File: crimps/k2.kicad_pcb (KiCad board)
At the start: 2 copper layers, 99 x 128.5 mm, 100 parts, among them IC1 TL074, IC2 TL072, IC3 TL074, J1 PJ301_THONKICONN6, J10 PJ301_THONKICONN6, J11 PJ301_THONKICONN6, J12 PJ301_THONKICONN6, J13 Conn_01x05_Female, J14 Conn_01x05_Female, J15 Conn_01x05_Female, J16 Conn_01x05_Male, J17 Conn_01x05_Male, J18 Conn_01x05_Male, J2 PJ301_THONKICONN6, J3 PJ301_THONKICONN6, J4 PJ301_THONKICONN6, J5 PJ301_THONKICONN6, J6 PJ301_THONKICONN6, J7 PJ301_THONKICONN6, J8 PJ301_THONKICONN6, J9 PJ301_THONKICONN6, Q1 MMBFJ309, Q2 MMBT3904, Q3 MMBT3904

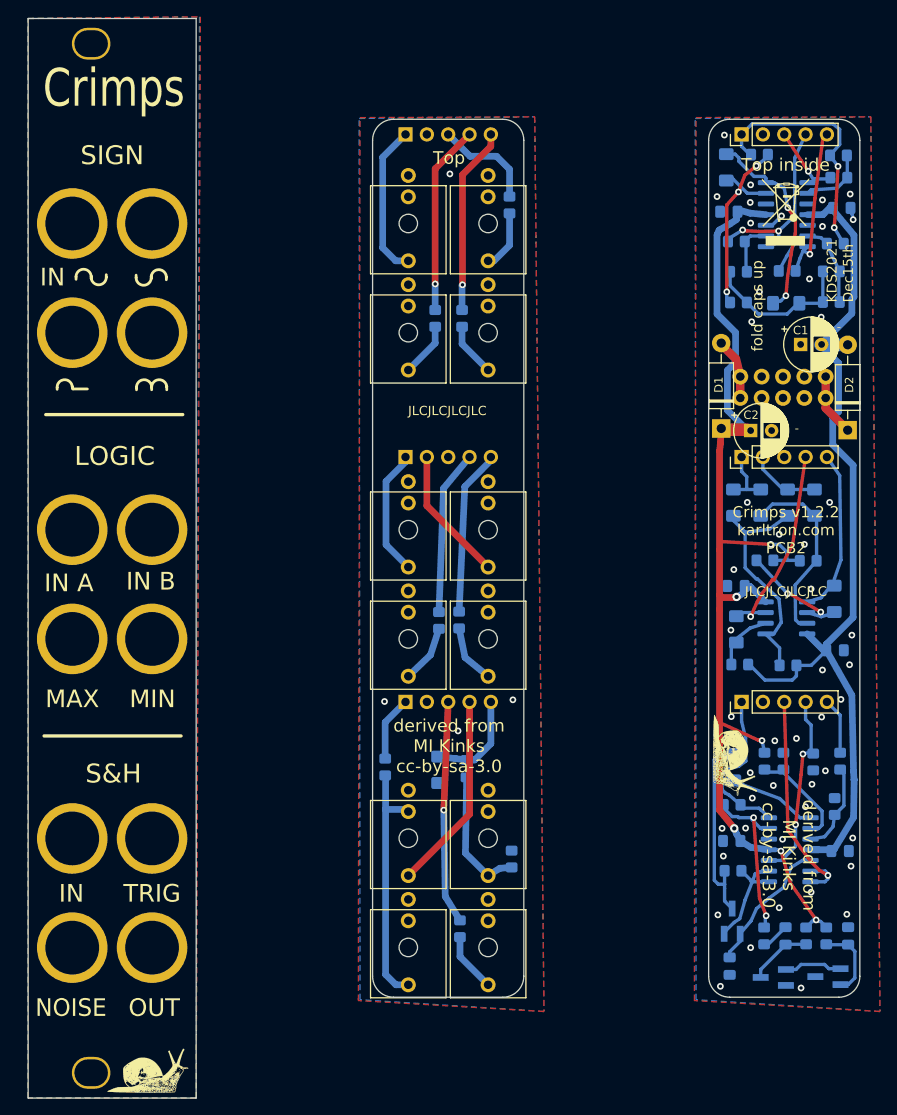
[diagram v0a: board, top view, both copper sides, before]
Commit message: update bom and version
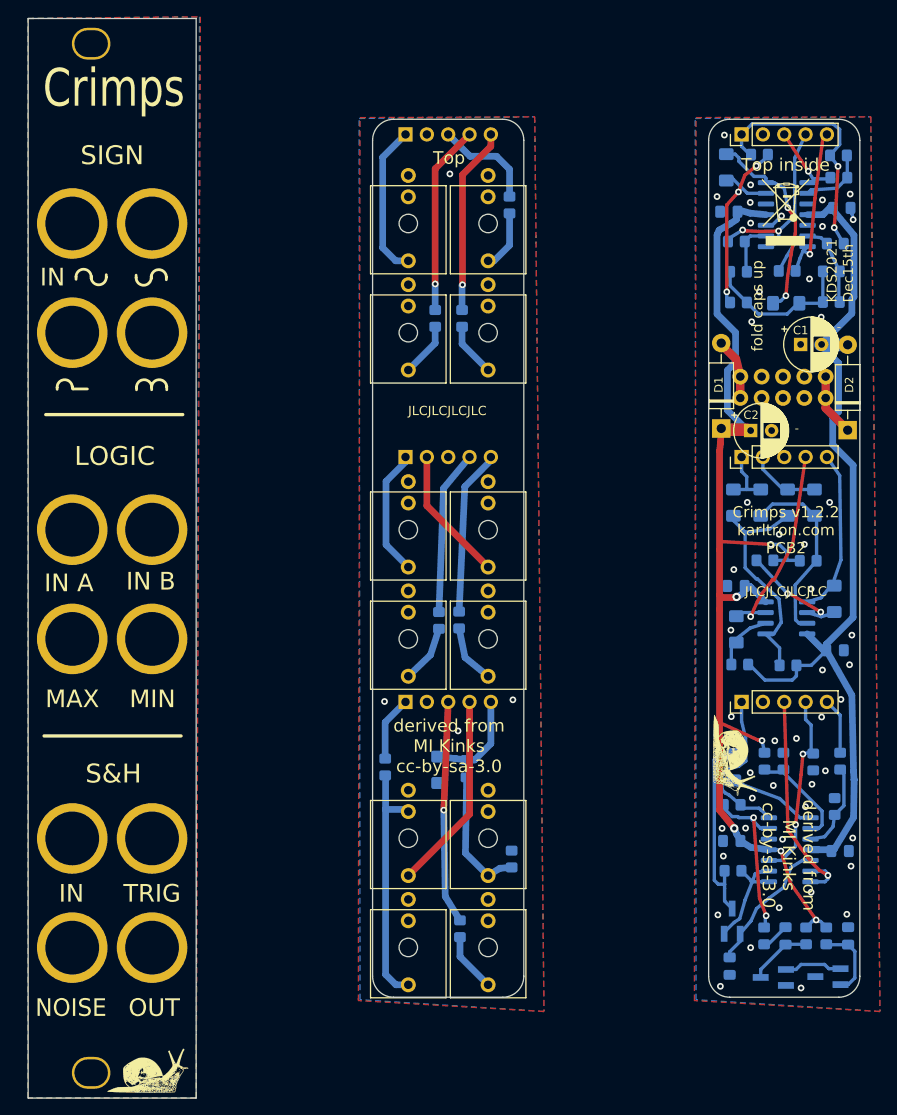
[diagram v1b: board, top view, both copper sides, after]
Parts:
- IC3: value TL074 -> OPA4171
- R27: value 1M -> 470K
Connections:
- J11 pad P2: (no net) -> unconnected-(J11-2-PadP2)
- J12 pad P2: (no net) -> unconnected-(J12-2-PadP2)
- J2 pad P2: (no net) -> unconnected-(J2-2-PadP2)
- J3 pad P2: (no net) -> unconnected-(J3-2-PadP2)
- J4 pad P2: (no net) -> unconnected-(J4-2-PadP2)
- J7 pad P2: (no net) -> unconnected-(J7-2-PadP2)
- J8 pad P2: (no net) -> unconnected-(J8-2-PadP2)
- Q2 pad 3: (no net) -> unconnected-(Q2-C-Pad3)
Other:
- net class Default removed
